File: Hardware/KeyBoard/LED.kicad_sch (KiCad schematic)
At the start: 101 parts

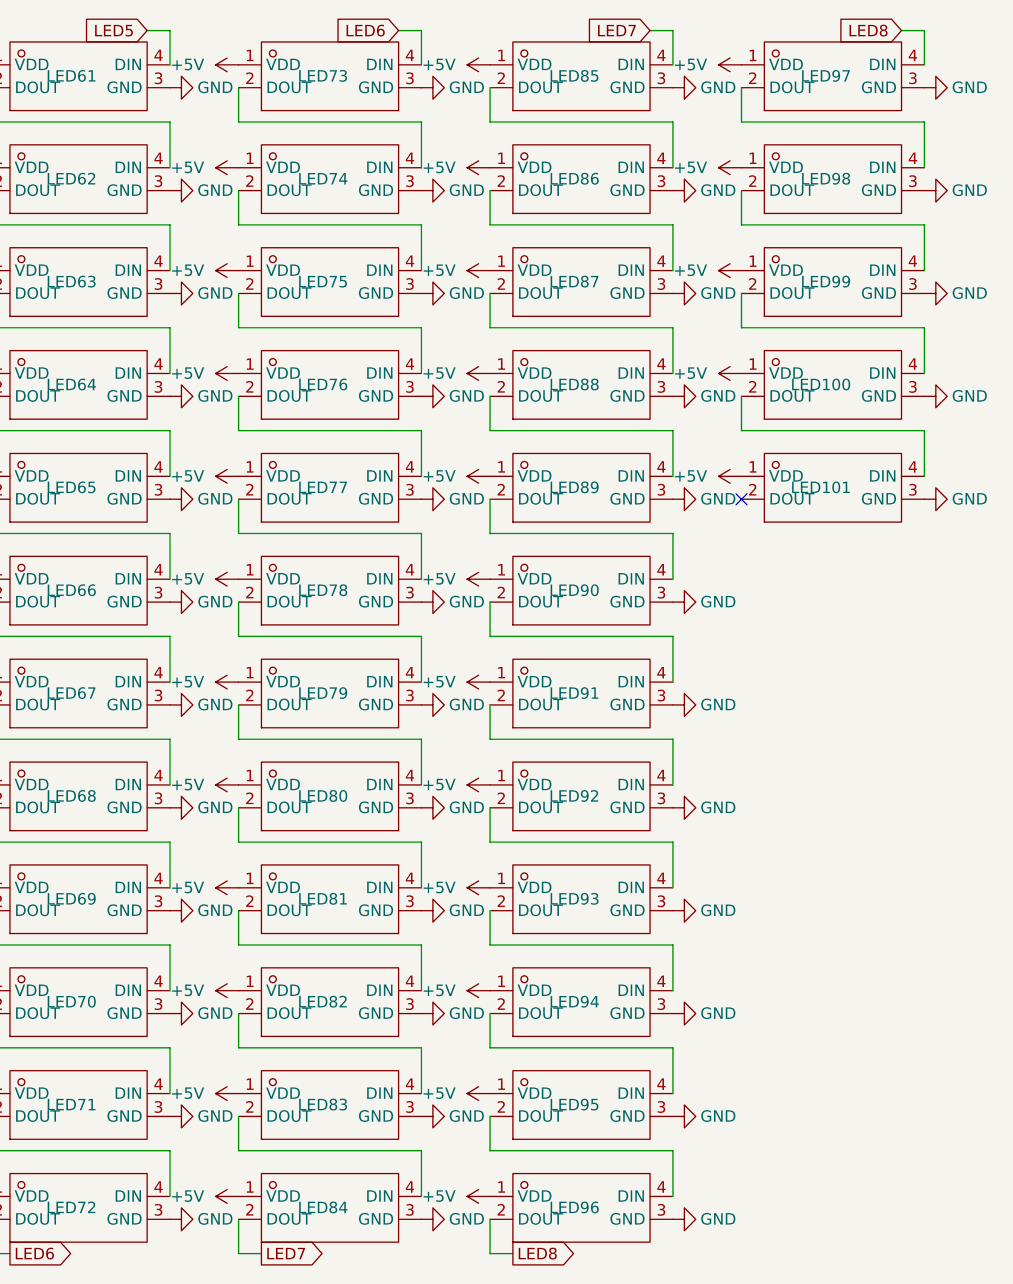
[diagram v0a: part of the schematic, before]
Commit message: complete layout
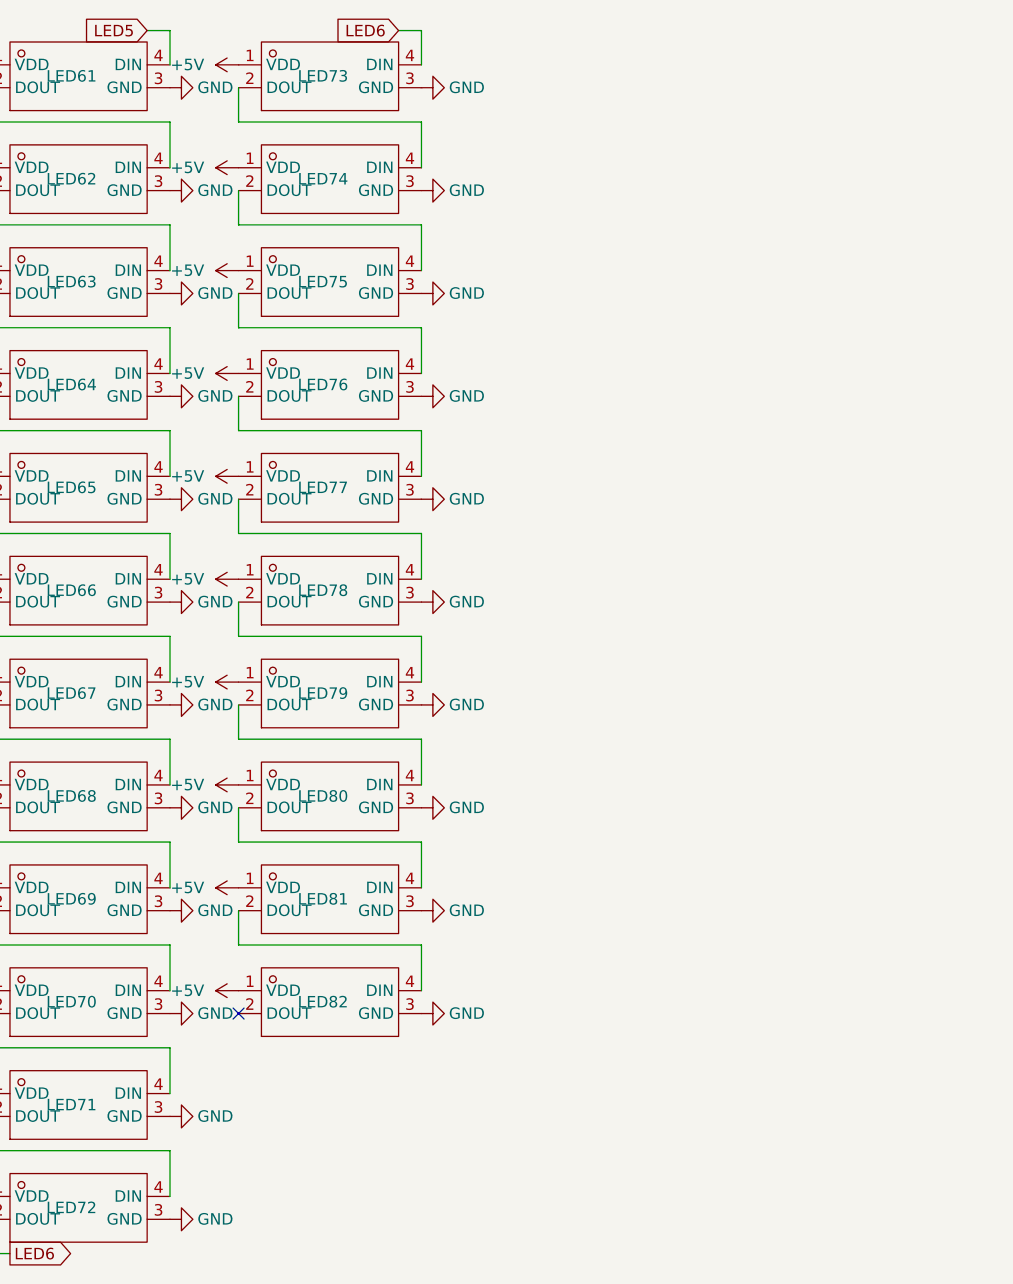
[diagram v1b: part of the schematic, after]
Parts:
- removed LED100, LED101, LED83, LED84, LED85, LED86, LED87, LED88, LED89, LED90, LED91, LED92, LED93, LED94, LED95, LED96, LED97, LED98, LED99: ~, persional_library:LED-SMD_L3.2-W2.8_YO-WS2812B-3528, symbol persional_library:YO-WS2812B-3528反贴
